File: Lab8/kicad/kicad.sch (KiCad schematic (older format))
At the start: 20 parts, among them U1 OPB745, U2 TLC277, U3 TLC277

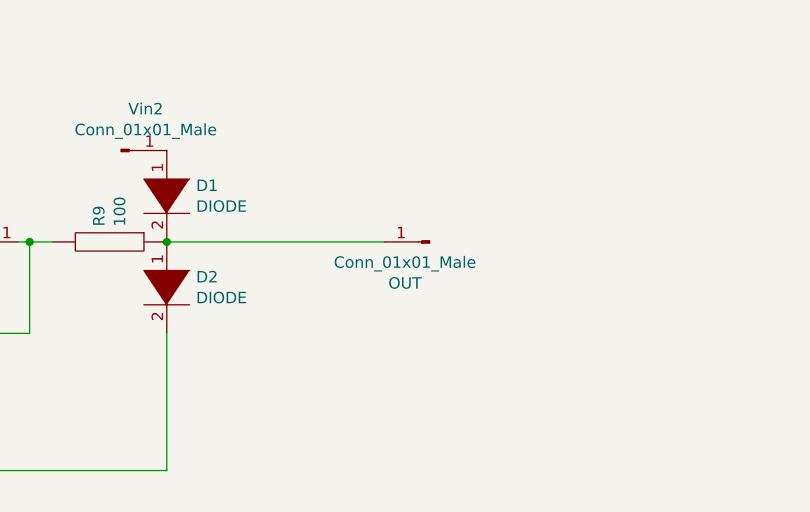
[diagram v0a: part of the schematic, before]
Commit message: some kicad stuff
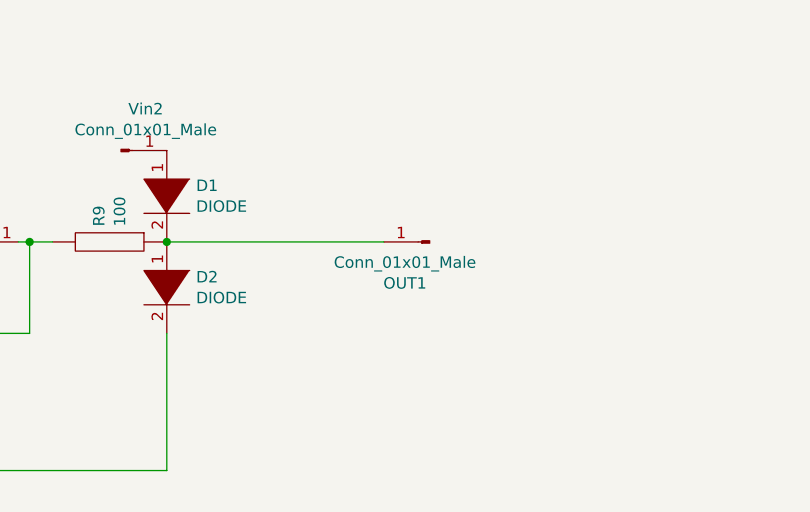
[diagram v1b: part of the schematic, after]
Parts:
- OUT1: renamed from OUT; footprint Connector_PinHeader_2.54mm:PinHeader_1x01_P2.54mm_Horizontal -> Connector_PinHeader_2.54mm:PinHeader_1x07_P2.54mm_Vertical_SMD_Pin1Left
- U1: footprint Connector_PinSocket_2.54mm:PinSocket_1x08_P2.54mm_Vertical -> Connector_PinHeader_2.54mm:PinHeader_1x04_P2.54mm_Vertical
- Vin1, Vin2: footprint Connector_PinHeader_2.54mm:PinHeader_1x01_P2.54mm_Horizontal -> Connector_PinHeader_2.54mm:PinHeader_1x08_P2.54mm_Vertical_SMD_Pin1Left
- gnd1: footprint Connector_PinHeader_2.54mm:PinHeader_1x01_P2.54mm_Horizontal -> Connector_PinHeader_2.54mm:PinHeader_1x07_P2.54mm_Vertical_SMD_Pin1Left
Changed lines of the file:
@@
-$EndComp
-$Comp
-L pspice:CAP C2
-U 1 1 61883FA3
-P 6150 3750
-F 0 "C2" V 5835 3750 50  0000 C CNN
-F 1 "97.3uf" V 5926 3750 50  0000 C CNN
-F 2 "Capacitor_SMD:CP_Elec_4x3" H 6150 3750 50  0001 C CNN
-F 3 "~" H 6150 3750 50  0001 C CNN
-	1    6150 3750
-	1    0    0    -1
 $EndComp
 $Comp
@@
 F 0 "Vin1" H 3308 2881 50  0000 C CNN
 F 1 "Conn_01x01_Male" H 3308 2790 50  0000 C CNN
-F 2 "Connector_PinHeader_2.54mm:PinHeader_1x01_P2.54mm_Horizontal" H 3200 2700 50  0001 C CNN
+F 2 "Connector_PinHeader_2.54mm:PinHeader_1x08_P2.54mm_Vertical_SMD_Pin1Left" H 3200 2700 50  0001 C CNN
 F 3 "~" H 3200 2700 50  0001 C CNN
 	1    3200 2700
@@
 F 0 "gnd1" V 5504 4462 50  0000 R CNN
 F 1 "Conn_01x01_Male" V 5413 4462 50  0000 R CNN
-F 2 "Connector_PinHeader_2.54mm:PinHeader_1x01_P2.54mm_Horizontal" H 5350 4550 50  0001 C CNN
+F 2 "Connector_PinHeader_2.54mm:PinHeader_1x07_P2.54mm_Vertical_SMD_Pin1Left" H 5350 4550 50  0001 C CNN
 F 3 "~" H 5350 4550 50  0001 C CNN
 	1    5350 4550
@@
 Wire Wire Line
 	6150 3350 6150 3500
-Connection ~ 6150 3350
-Wire Wire Line
-	6150 3350 6450 3350
-$Comp
-L Amplifier_Operational:TLC277 U3
-U 1 1 61881D6C
-P 6750 3450
-F 0 "U3" H 6750 3817 50  0000 C CNN
-F 1 "TLC277" H 6750 3726 50  0000 C CNN
-F 2 "TLC277CP:DIP794W45P254L959H508Q8" H 6750 3450 50  0001 C CNN
-F 3 "http://www.ti.com/lit/ds/symlink/tlc272.pdf" H 6750 3450 50  0001 C CNN
-	1    6750 3450
-	1    0    0    -1
-$EndComp
 Wire Wire Line
 	6950 3850 7100 3850
@@
 F 0 "U1" H 4028 2496 50  0000 L CNN
 F 1 "OPB745" H 4028 2405 50  0000 L CNN
-F 2 "Connector_PinSocket_2.54mm:PinSocket_1x08_P2.54mm_Vertical" H 2800 3350 50  0001 L CNN
+F 2 "Connector_PinHeader_2.54mm:PinHeader_1x04_P2.54mm_Vertical" H 2800 3350 50  0001 L CNN
 F 3 "https://upverter.com/datasheet/4f8d3d5f99316b04551580b4d6f54087dceae820.pdf" H 2800 3450 50  0001 L CNN
 F 4 "IC" H 2800 3550 50  0001 L CNN "category"
@@
 F 0 "Vin2" H 7608 3231 50  0000 C CNN
 F 1 "Conn_01x01_Male" H 7608 3140 50  0000 C CNN
-F 2 "Connector_PinHeader_2.54mm:PinHeader_1x01_P2.54mm_Horizontal" H 7500 3050 50  0001 C CNN
+F 2 "Connector_PinHeader_2.54mm:PinHeader_1x08_P2.54mm_Vertical_SMD_Pin1Left" H 7500 3050 50  0001 C CNN
 F 3 "~" H 7500 3050 50  0001 C CNN
 	1    7500 3050
@@
 	6400 3950 6400 3850
 Wire Wire Line
-	6400 3550 6450 3550
-Wire Wire Line
 	6450 3850 6400 3850
-Connection ~ 6400 3850
-Wire Wire Line
-	6400 3850 6400 3550
-$Comp
-L Connector:Conn_01x01_Male OUT
+$Comp
+L Connector:Conn_01x01_Male OUT1
 U 1 1 6193298D
 P 8850 3450
-F 0 "OUT" H 8958 3631 50  0000 C CNN
+F 0 "OUT1" H 8958 3631 50  0000 C CNN
 F 1 "Conn_01x01_Male" H 8958 3540 50  0000 C CNN
-F 2 "Connector_PinHeader_2.54mm:PinHeader_1x01_P2.54mm_Horizontal" H 8850 3450 50  0001 C CNN
+F 2 "Connector_PinHeader_2.54mm:PinHeader_1x07_P2.54mm_Vertical_SMD_Pin1Left" H 8850 3450 50  0001 C CNN
 F 3 "~" H 8850 3450 50  0001 C CNN
 	1    8850 3450
@@
 Wire Wire Line
 	7700 3450 8650 3450
+Connection ~ 6400 3850
+Connection ~ 6150 3350
+Wire Wire Line
+	6400 3850 6400 3550
+Wire Wire Line
+	6400 3550 6450 3550
+Wire Wire Line
+	6150 3350 6450 3350
+$Comp
+L pspice:CAP C2
+U 1 1 61883FA3
+P 6150 3750
+F 0 "C2" V 5835 3750 50  0000 C CNN
+F 1 "97.3uf" V 5926 3750 50  0000 C CNN
+F 2 "Capacitor_SMD:CP_Elec_4x3" H 6150 3750 50  0001 C CNN
+F 3 "~" H 6150 3750 50  0001 C CNN
+	1    6150 3750
+	1    0    0    -1
+$EndComp
+$Comp
+L Amplifier_Operational:TLC277 U3
+U 1 1 61881D6C
+P 6750 3450
+F 0 "U3" H 6750 3817 50  0000 C CNN
+F 1 "TLC277" H 6750 3726 50  0000 C CNN
+F 2 "TLC277CP:DIP794W45P254L959H508Q8" H 6750 3450 50  0001 C CNN
+F 3 "http://www.ti.com/lit/ds/symlink/tlc272.pdf" H 6750 3450 50  0001 C CNN
+	1    6750 3450
+	1    0    0    -1
+$EndComp
 $EndSCHEMATC
